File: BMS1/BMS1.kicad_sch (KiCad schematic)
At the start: 68 parts, among them J1 Conn_01x02, Q1 Q_NPN_BCE, Q2 Q_NPN_BCE, T1 ESMIT-4180_C, U1 ADG728, U10 LTC6812-1, U2 ADG728, U3 ADG728, U4 ADG728, U5 ADG728, U6 ADG728, U7 ADG728, U8 ADG728, U9 LTC6812-1

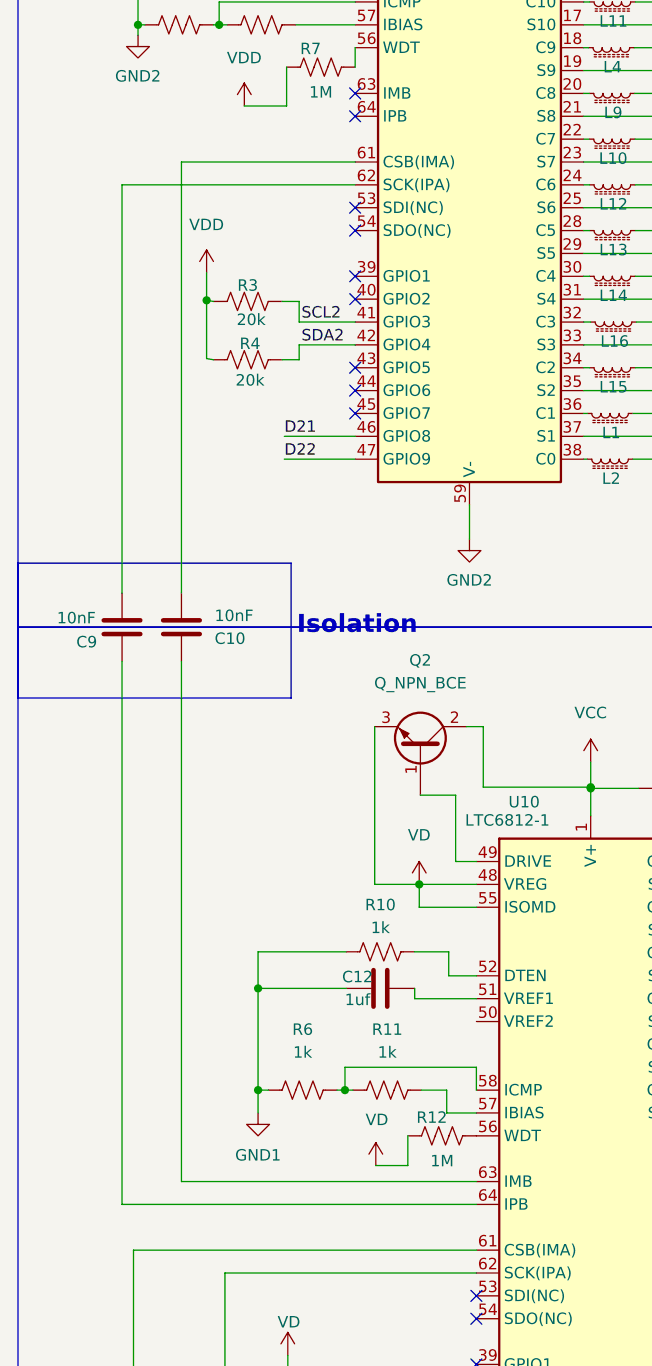
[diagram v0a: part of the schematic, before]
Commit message: Cap Change
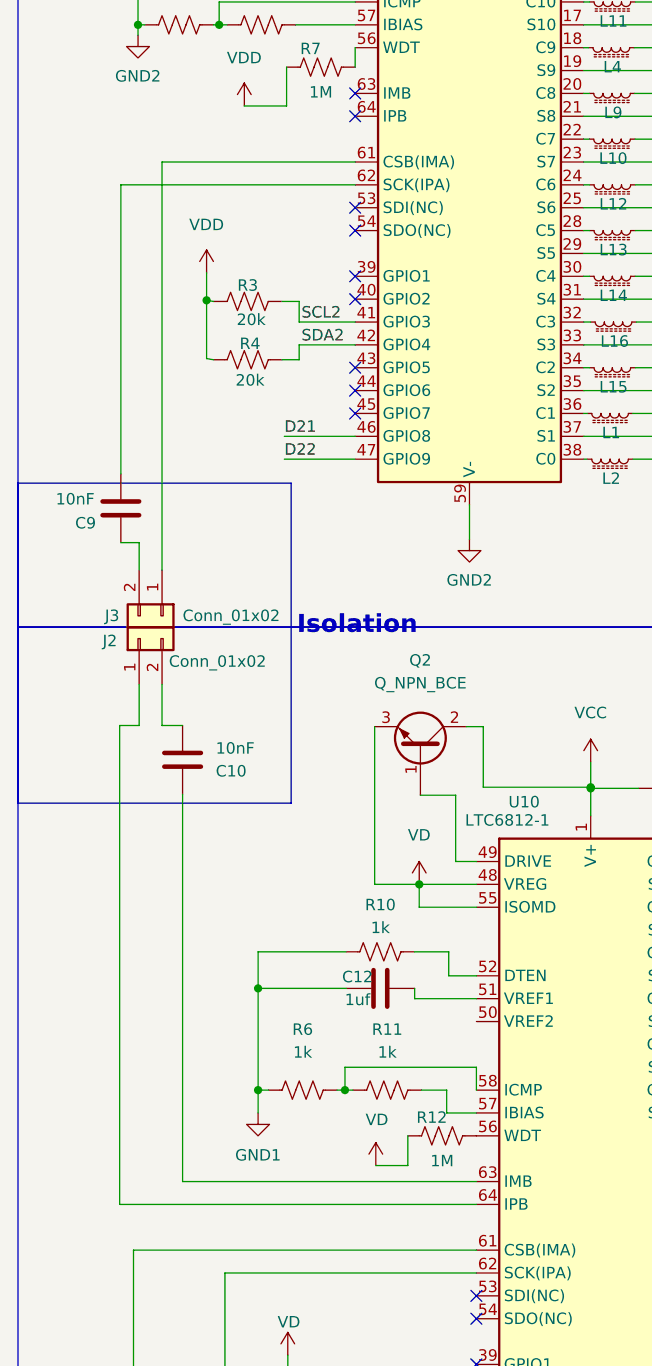
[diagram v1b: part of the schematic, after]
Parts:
- added J2, J3: Conn_01x02, Connector_JST:JST_XH_B2B-XH-A_1x02_P2.50mm_Vertical, symbol Connector_Generic:Conn_01x02
- C10, C9: footprint Capacitor_SMD:C_0603_1608Metric_Pad1.08x0.95mm_HandSolder -> Capacitor_SMD:C_0805_2012Metric_Pad1.18x1.45mm_HandSolder
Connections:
- net at C9.2: now also J3.2 (Pin_2); no longer U10.64 (IPB)
- net at C10.1: now also J2.2 (Pin_2); no longer U9.61 (CSB(IMA))
- new net: J2.1 (Pin_1), U10.64 (IPB)
- new net: J3.1 (Pin_1), U9.61 (CSB(IMA))
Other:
- moved on the sheet: C10, C9
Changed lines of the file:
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@@
     (stroke (width 0) (type default))
   )
-  (wire (pts (xy 28.321 196.977) (xy 67.697 196.977))
+  (wire (pts (xy 54.229 70.612) (xy 54.229 68.453))
     (stroke (width 0) (type default))
   )
-  (wire (pts (xy 54.229 70.612) (xy 54.229 68.453))
+  (wire (pts (xy 28.194 123.444) (xy 30.226 123.444))
+    (stroke (width 0) (type default))
+  )
+  (wire (pts (xy 32.766 81.153) (xy 54.229 81.153))
     (stroke (width 0) (type default))
   )
@@
     (stroke (width 0) (type default))
   )
+  (wire (pts (xy 30.226 123.444) (xy 30.226 126.492))
+    (stroke (width 0) (type default))
+  )
   (wire (pts (xy 253.746 119.888) (xy 254.381 119.888))
     (stroke (width 0) (type default))
@@
     (stroke (width 0) (type default))
   )
+  (wire (pts (xy 30.226 139.192) (xy 30.226 143.764))
+    (stroke (width 0) (type default))
+  )
   (wire (pts (xy 260.604 44.704) (xy 269.24 44.704))
     (stroke (width 0) (type default))
@@
     (stroke (width 0) (type default))
   )
+  (wire (pts (xy 35.052 143.764) (xy 32.766 143.764))
+    (stroke (width 0) (type default))
+  )
   (wire (pts (xy 213.868 224.917) (xy 213.868 227.457))
     (stroke (width 0) (type default))
@@
     (stroke (width 0) (type default))
   )
-  (wire (pts (xy 34.925 194.437) (xy 67.697 194.437))
+  (wire (pts (xy 35.052 194.437) (xy 67.697 194.437))
     (stroke (width 0) (type default))
   )
@@
     (stroke (width 0) (type default))
   )
-  (wire (pts (xy 28.321 136.652) (xy 28.321 196.977))
-    (stroke (width 0) (type default))
-  )
   (bus (pts (xy 126.498 169.037) (xy 126.498 166.497))
     (stroke (width 0) (type default))
@@
     (stroke (width 0) (type default))
   )
+  (wire (pts (xy 30.226 143.764) (xy 28.061 143.764))
+    (stroke (width 0) (type default))
+  )
   (wire (pts (xy 65.3933 151.511) (xy 61.474 151.511))
     (stroke (width 0) (type default))
@@
     (stroke (width 0) (type default))
   )
+  (wire (pts (xy 28.061 196.977) (xy 67.697 196.977))
+    (stroke (width 0) (type default))
+  )
   (wire (pts (xy 273.304 187.96) (xy 274.955 187.96))
     (stroke (width 0) (type default))
@@
     (stroke (width 0) (type default))
   )
-  (wire (pts (xy 28.321 83.693) (xy 28.321 129.032))
+  (wire (pts (xy 28.194 83.693) (xy 28.194 115.824))
     (stroke (width 0) (type default))
   )
@@
     (stroke (width 0) (type default))
   )
-  (wire (pts (xy 34.925 136.652) (xy 34.925 194.437))
+  (wire (pts (xy 32.766 126.492) (xy 32.766 81.153))
+    (stroke (width 0) (type default))
+  )
+  (wire (pts (xy 35.052 151.384) (xy 35.052 194.437))
     (stroke (width 0) (type default))
   )
@@
     (stroke (width 0) (type default))
   )
-  (wire (pts (xy 34.925 81.153) (xy 34.925 129.032))
-    (stroke (width 0) (type default))
-  )
   (wire (pts (xy 251.46 245.237) (xy 245.237 245.237))
     (stroke (width 0) (type default))
@@
     (stroke (width 0) (type default))
   )
-  (wire (pts (xy 54.229 83.693) (xy 28.321 83.693))
+  (wire (pts (xy 54.229 83.693) (xy 28.194 83.693))
     (stroke (width 0) (type default))
   )
@@
     (stroke (width 0) (type default))
   )
-  (wire (pts (xy 54.229 81.153) (xy 34.925 81.153))
-    (stroke (width 0) (type default))
-  )
   (wire (pts (xy 79.629 86.233) (xy 107.569 86.233))
     (stroke (width 0) (type default))
@@
     (stroke (width 0) (type default))
   )
+  (wire (pts (xy 28.061 143.764) (xy 28.061 196.977))
+    (stroke (width 0) (type default))
+  )
   (wire (pts (xy 253.619 60.452) (xy 253.619 61.976))
     (stroke (width 0) (type default))
@@
     (stroke (width 0) (type default))
   )
+  (wire (pts (xy 32.766 143.764) (xy 32.766 139.192))
+    (stroke (width 0) (type default))
+  )
   (wire (pts (xy 267.208 59.944) (xy 272.796 59.944))
     (stroke (width 0) (type default))
@@
     (fill (type none))
   )
-  (rectangle (start 16.764 125.73) (end 47.117 140.716)
+  (rectangle (start 16.764 116.84) (end 47.117 152.4)
     (stroke (width 0) (type default))
     (fill (type none))
@@
     )
   )
-  (symbol (lib_id "Device:C") (at 28.321 132.842 0) (unit 1)
+  (symbol (lib_id "Device:C") (at 28.194 119.634 0) (unit 1)
     (in_bom yes) (on_board yes) (dnp no)
-    (property "Reference" "C9" (at 23.241 134.493 0)
+    (property "Reference" "C9" (at 23.114 121.285 0)
       (effects (font (size 1.27 1.27)) (justify left))
     )
-    (property "Value" "10nF" (at 21.082 131.826 0)
+    (property "Value" "10nF" (at 20.955 118.618 0)
       (effects (font (size 1.27 1.27)) (justify left))
     )
-    (property "Footprint" "Capacitor_SMD:C_0603_1608Metric_Pad1.08x0.95mm_HandSolder" (at 29.2862 136.652 0)
+    (property "Footprint" "Capacitor_SMD:C_0805_2012Metric_Pad1.18x1.45mm_HandSolder" (at 29.1592 123.444 0)
       (effects (font (size 1.27 1.27)) hide)
     )
-    (property "Datasheet" "~" (at 28.321 132.842 0)
+    (property "Datasheet" "~" (at 28.194 119.634 0)
       (effects (font (size 1.27 1.27)) hide)
     )
@@
     )
   )
+  (symbol (lib_id "Connector_Generic:Conn_01x02") (at 30.226 134.112 90) (unit 1)
+    (in_bom yes) (on_board yes) (dnp no)
+    (property "Reference" "J2" (at 26.162 134.366 90)
+      (effects (font (size 1.27 1.27)) (justify right))
+    )
+    (property "Value" "Conn_01x02" (at 33.528 136.652 90)
+      (effects (font (size 1.27 1.27)) (justify right))
+    )
+    (property "Footprint" "Connector_JST:JST_XH_B2B-XH-A_1x02_P2.50mm_Vertical" (at 30.226 134.112 0)
+      (effects (font (size 1.27 1.27)) hide)
+    )
+    (property "Datasheet" "~" (at 30.226 134.112 0)
+      (effects (font (size 1.27 1.27)) hide)
+    )
+    (pin "1")
+    (pin "2")
+    (instances
+      (project "BMS1"
+        (path "/03933f33-7fdb-43de-9d7d-a565cad8a277"
+          (reference "J2") (unit 1)
+        )
+      )
+    )
+  )
   (symbol (lib_id "Connector_Generic:Conn_01x02") (at 36.074 257.81 270) (unit 1)
     (in_bom yes) (on_board yes) (dnp no) (fields_autoplaced)
@@
     )
   )
+  (symbol (lib_id "Connector_Generic:Conn_01x02") (at 32.766 131.572 270) (unit 1)
+    (in_bom yes) (on_board yes) (dnp no)
+    (property "Reference" "J3" (at 26.416 131.572 90)
+      (effects (font (size 1.27 1.27)) (justify left))
+    )
+    (property "Value" "Conn_01x02" (at 35.052 131.572 90)
+      (effects (font (size 1.27 1.27)) (justify left))
+    )
+    (property "Footprint" "Connector_JST:JST_XH_B2B-XH-A_1x02_P2.50mm_Vertical" (at 32.766 131.572 0)
+      (effects (font (size 1.27 1.27)) hide)
+    )
+    (property "Datasheet" "~" (at 32.766 131.572 0)
+      (effects (font (size 1.27 1.27)) hide)
+    )
+    (pin "1")
+    (pin "2")
+    (instances
+      (project "BMS1"
+        (path "/03933f33-7fdb-43de-9d7d-a565cad8a277"
+          (reference "J3") (unit 1)
+        )
+      )
+    )
+  )
   (symbol (lib_id "power:VDD") (at 222.885 95.377 0) (unit 1)
     (in_bom yes) (on_board yes) (dnp no) (fields_autoplaced)
@@
     )
   )
-  (symbol (lib_id "Device:C") (at 34.925 132.842 0) (unit 1)
+  (symbol (lib_id "Device:C") (at 35.052 147.574 0) (unit 1)
     (in_bom yes) (on_board yes) (dnp no)
-    (property "Reference" "C10" (at 38.608 134.112 0)
+    (property "Reference" "C10" (at 38.735 148.844 0)
       (effects (font (size 1.27 1.27)) (justify left))
     )
-    (property "Value" "10nF" (at 38.608 131.572 0)
+    (property "Value" "10nF" (at 38.735 146.304 0)
       (effects (font (size 1.27 1.27)) (justify left))
     )
-    (property "Footprint" "Capacitor_SMD:C_0603_1608Metric_Pad1.08x0.95mm_HandSolder" (at 35.8902 136.652 0)
+    (property "Footprint" "Capacitor_SMD:C_0805_2012Metric_Pad1.18x1.45mm_HandSolder" (at 36.0172 151.384 0)
       (effects (font (size 1.27 1.27)) hide)
     )
-    (property "Datasheet" "~" (at 34.925 132.842 0)
+    (property "Datasheet" "~" (at 35.052 147.574 0)
       (effects (font (size 1.27 1.27)) hide)
     )
